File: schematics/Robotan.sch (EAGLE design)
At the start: 9 parts, among them U1 MAX232PTH

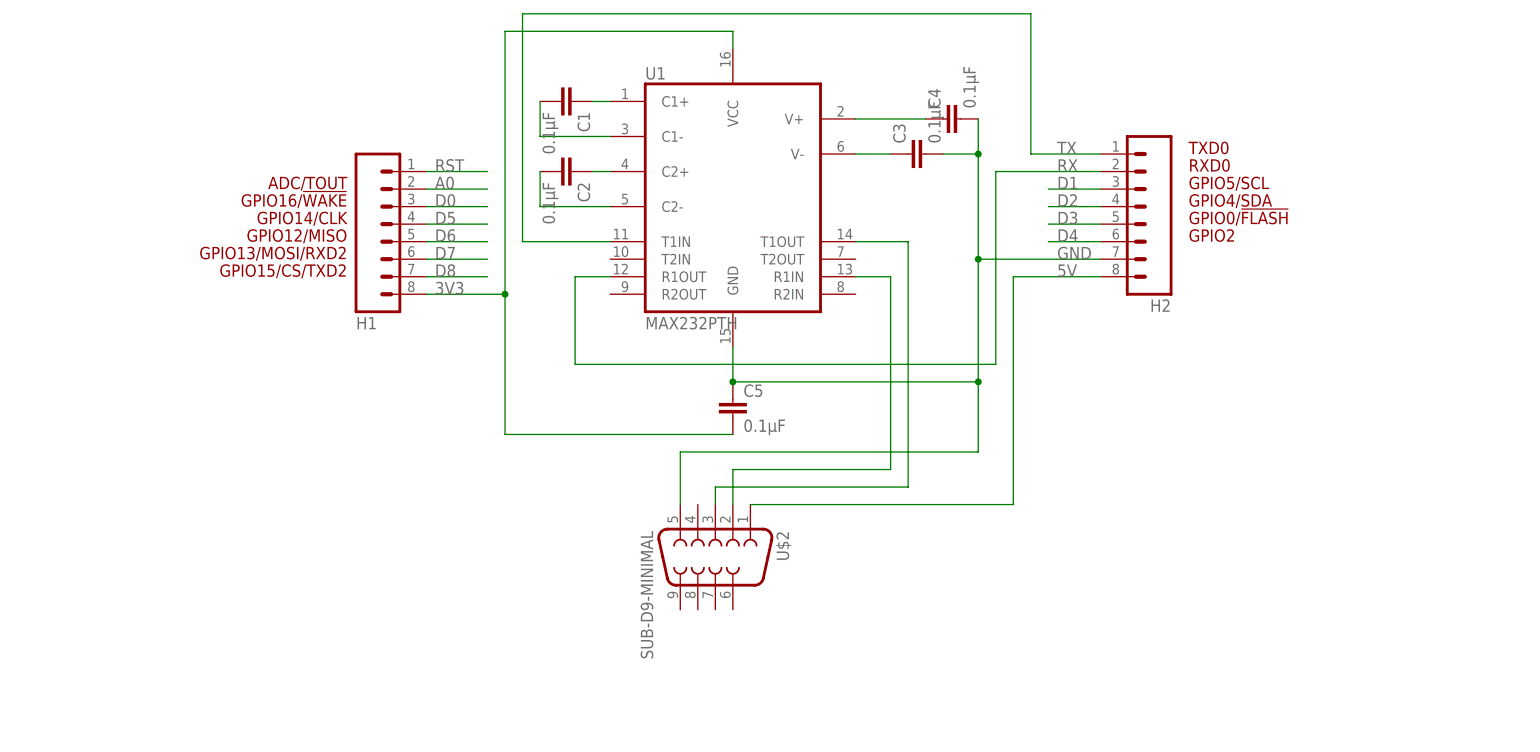
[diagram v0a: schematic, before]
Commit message: New board layout
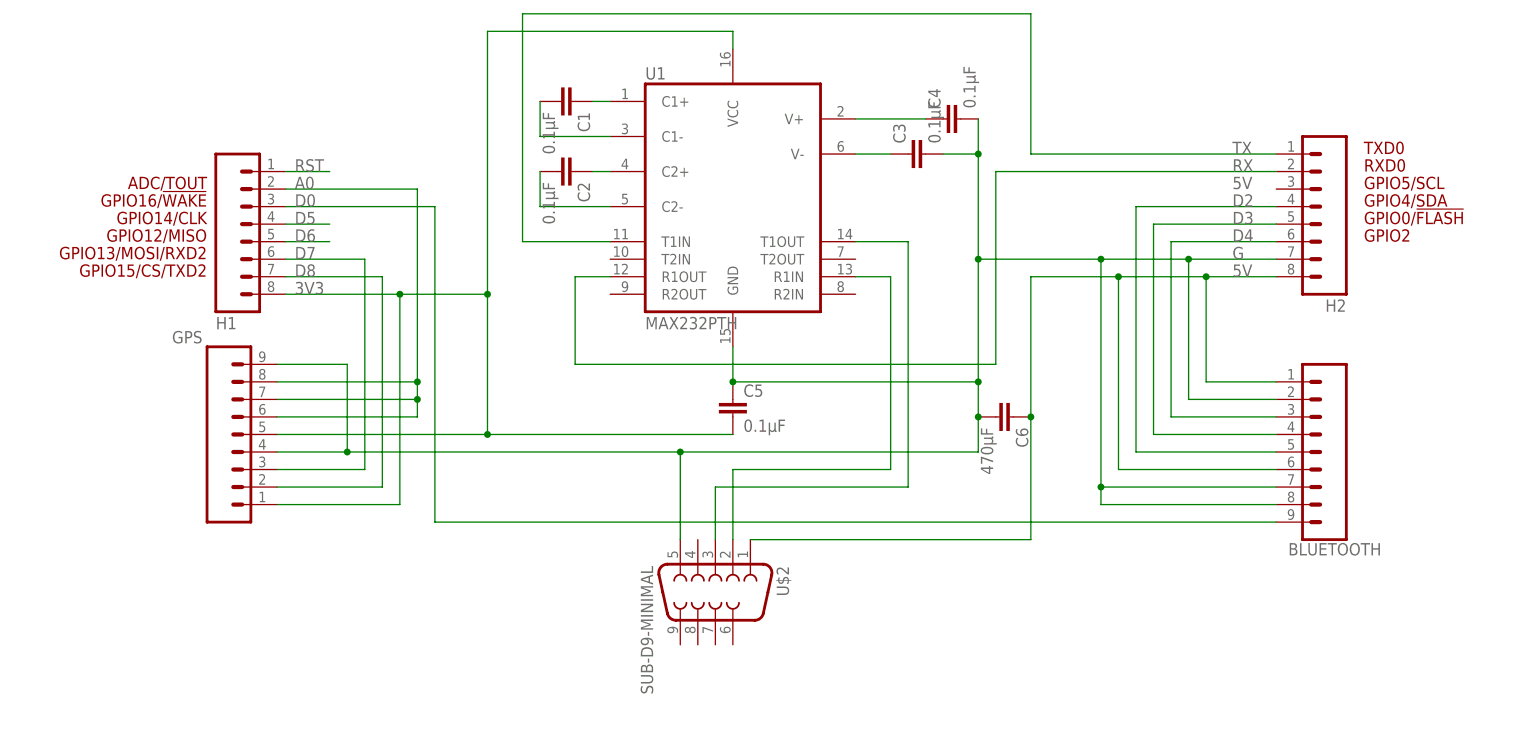
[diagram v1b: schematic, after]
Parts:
- added BLUETOOTH, GPS: (no value), SparkFun-Connectors:M09
- added C6: 470µF, SparkFun-Capacitors:0.1UF-50V-20%(PTH)KIT-EZ
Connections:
- removed net D1: H2.3
- removed net GND: C3.2, C4.2, C5.1, H2.7, U$2.5, U1.GND
- new net G: BLUETOOTH.2, BLUETOOTH.7, BLUETOOTH.8, C3.2, C4.2, C5.1, C6.2, GPS.4, GPS.9, H2.7, U$2.5, U1.GND
- net 3V3: now also GPS.1, GPS.5
- net 5V: now also BLUETOOTH.1, BLUETOOTH.6, C6.1
- net A0: now also GPS.6, GPS.7, GPS.8
- net D0: now also BLUETOOTH.9
- net D2: now also BLUETOOTH.5
- net D3: now also BLUETOOTH.4
- net D4: now also BLUETOOTH.3
- net D7: now also GPS.3
- net D8: now also GPS.2
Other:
- moved on the sheet: H1, H2, U$2
